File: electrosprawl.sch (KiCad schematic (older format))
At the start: 53 parts, among them J1 3.3v, J2 Conn_02x08_Odd_Even, J67 Conn_02x05_Counter_Clockwise, J7 VCC, J70 TXRX, J71 Micro_SD_Card_Det, J74 USB_B_Micro, SW1 Reset, U2 samd51p20, U5 LM1117-3.3, Y1 Crystal

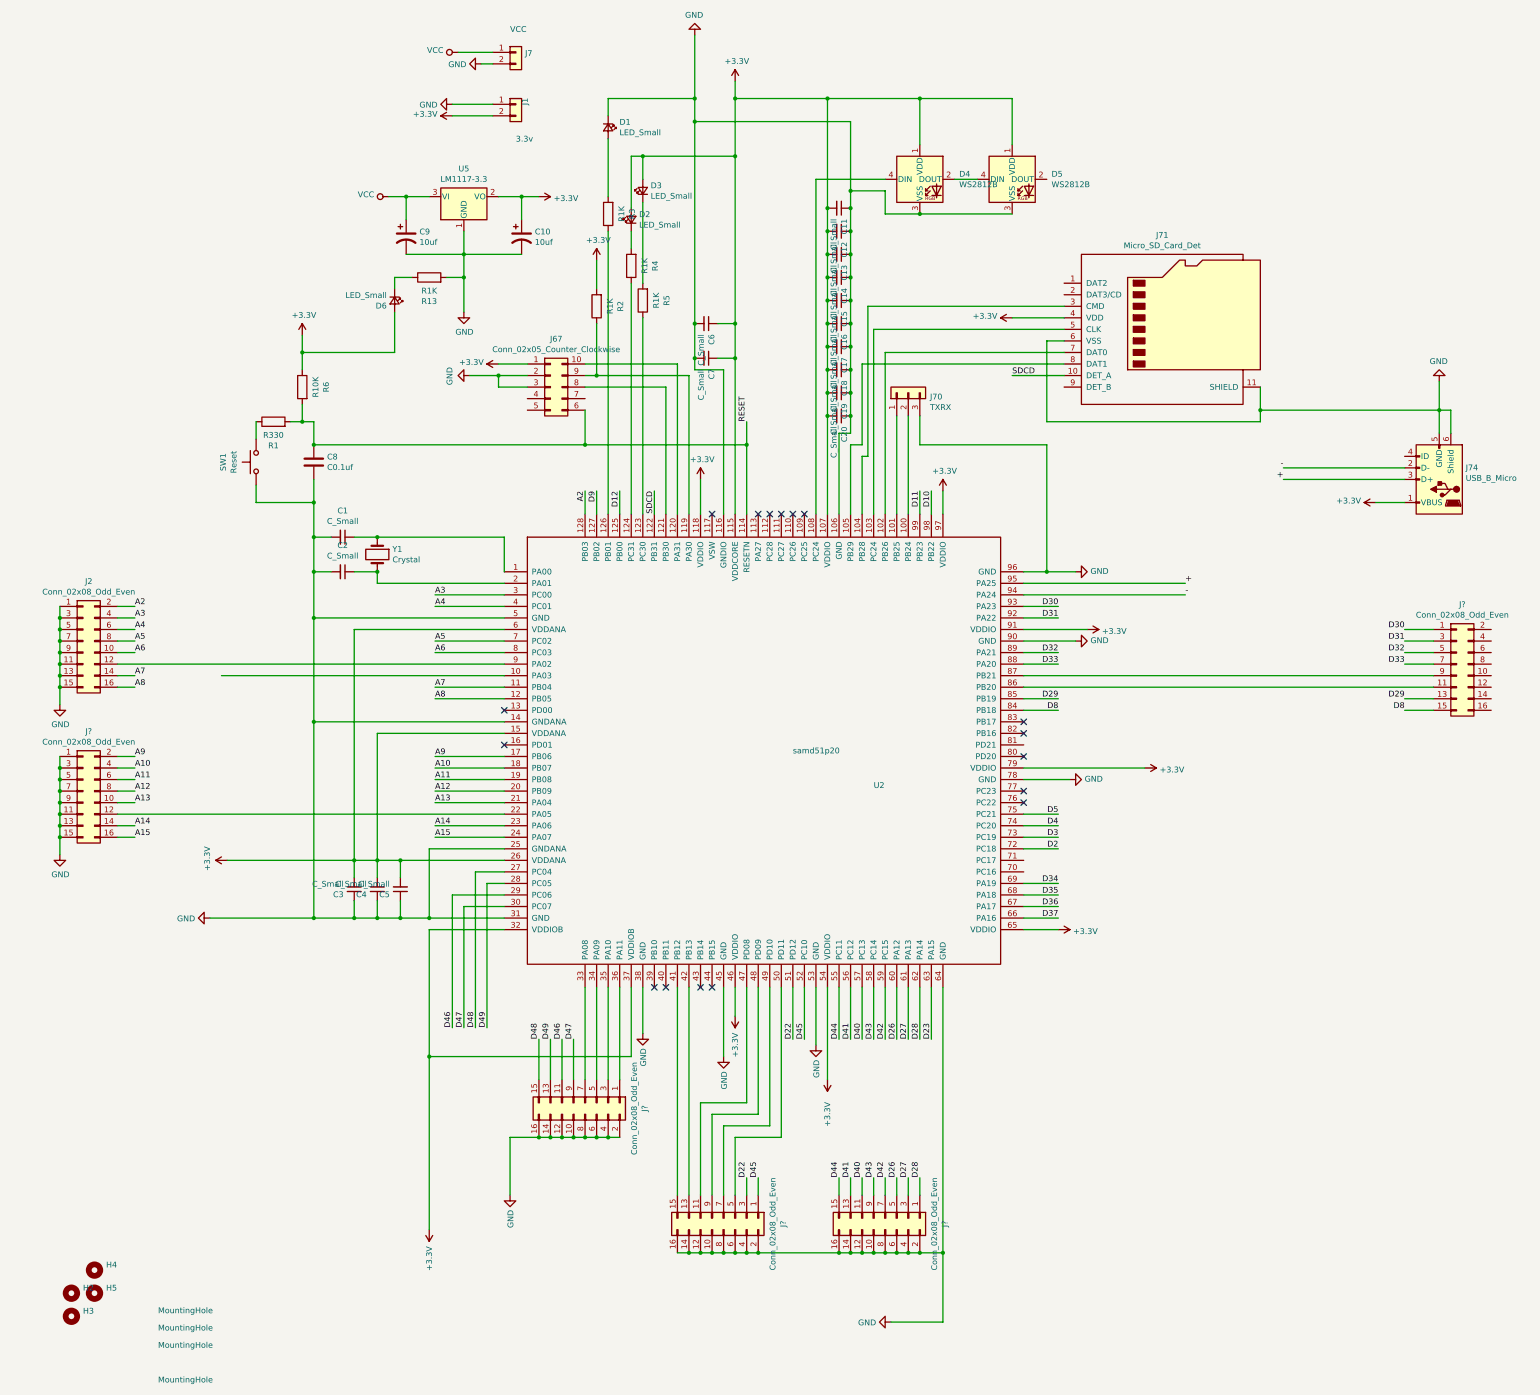
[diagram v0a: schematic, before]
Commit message: update layout
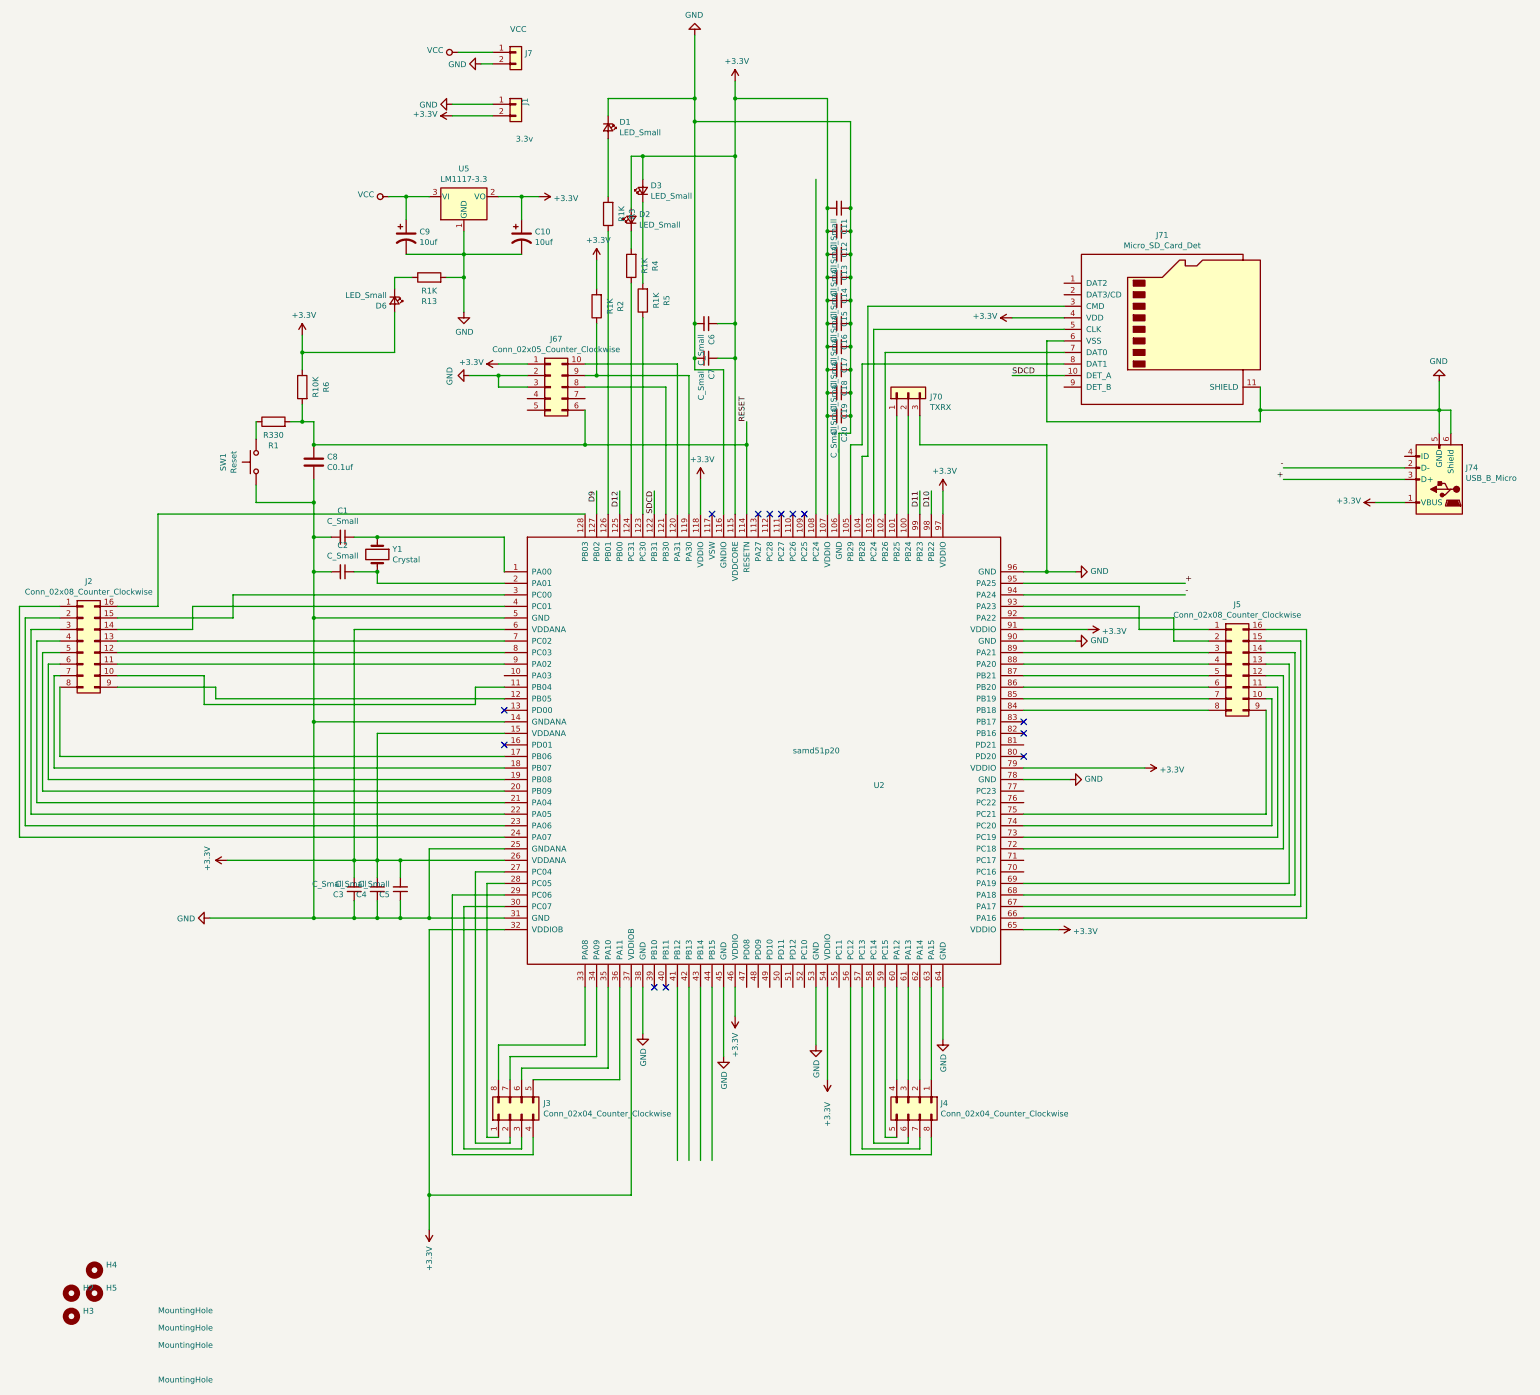
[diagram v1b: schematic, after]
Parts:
- removed D4, D5: WS2812B, LED_SMD:LED_WS2812B_PLCC4_5.0x5.0mm_P3.2mm, symbol LED:WS2812B
- removed J2, J? (x5): Conn_02x08_Odd_Even, Connector_PinHeader_2.54mm:PinHeader_2x08_P2.54mm_Vertical, symbol Connector_Generic:Conn_02x08_Odd_Even
- added J2, J5: Conn_02x08_Counter_Clockwise, Connector_PinHeader_2.54mm:PinHeader_2x08_P2.54mm_Vertical, symbol Connector_Generic:Conn_02x08_Counter_Clockwise
- added J3, J4: Conn_02x04_Counter_Clockwise, Connector_PinHeader_2.54mm:PinHeader_2x04_P2.54mm_Vertical, symbol Connector_Generic:Conn_02x04_Counter_Clockwise
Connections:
- net at U2.22 (PA05): now also J2.3 (Pin_3)
- net at U2.33 (PA08): now also J3.8 (Pin_8)
- net at U2.34 (PA09): now also J3.7 (Pin_7)
- net at U2.35 (PA10): now also J3.6 (Pin_6)
- net at U2.36 (PA11): now also J3.5 (Pin_5)
- net at U2.86 (PB20): now also J5.6 (Pin_6)
- net at U2.87 (PB21): now also J5.5 (Pin_5)
- net at U2.9 (PA02): now also J2.11 (Pin_11)
- net A10: no longer names the net of U2.18 (PB07)
- net A10: now also J2.7 (Pin_7)
- net A11: no longer names the net of U2.19 (PB08)
- net A11: now also J2.6 (Pin_6)
- net A12: no longer names the net of U2.20 (PB09)
- net A12: now also J2.5 (Pin_5)
- net A13: no longer names the net of U2.21 (PA04)
- net A13: now also J2.4 (Pin_4)
- net A14: no longer names the net of U2.23 (PA06)
- net A14: now also J2.2 (Pin_2)
- net A15: no longer names the net of U2.24 (PA07)
- net A15: now also J2.1 (Pin_1)
- net A2: no longer names the net of U2.128 (PB03)
- net A2: now also J2.16 (Pin_16)
- net A3: no longer names the net of U2.3 (PC00)
- net A3: now also J2.15 (Pin_15)
- net A4: no longer names the net of U2.4 (PC01)
- net A4: now also J2.14 (Pin_14)
- net A5: no longer names the net of U2.7 (PC02)
- net A5: now also J2.13 (Pin_13)
- net A6: no longer names the net of U2.8 (PC03)
- net A6: now also J2.12 (Pin_12)
- net A7: no longer names the net of U2.11 (PB04)
- net A7: now also J2.10 (Pin_10)
- net A8: no longer names the net of U2.12 (PB05)
- net A8: now also J2.9 (Pin_9)
- net A9: no longer names the net of U2.17 (PB06)
- net A9: now also J2.8 (Pin_8)
- net D2: no longer names the net of U2.72 (PC18)
- net D2: now also J5.12 (Pin_12)
- net D22: no longer names the net of U2.51 (PD12)
- net D23: no longer names the net of U2.63 (PA15)
- net D23: now also J4.1 (Pin_1)
- net D26: no longer names the net of U2.60 (PA12)
- net D26: now also J4.4 (Pin_4)
- net D27: no longer names the net of U2.61 (PA13)
- net D27: now also J4.3 (Pin_3)
- net D28: no longer names the net of U2.62 (PA14)
- net D28: now also J4.2 (Pin_2)
- net D29: no longer names the net of U2.85 (PB19)
- net D29: now also J5.7 (Pin_7)
- net D3: no longer names the net of U2.73 (PC19)
- net D3: now also J5.11 (Pin_11)
- net D30: no longer names the net of U2.93 (PA23)
- net D30: now also J5.1 (Pin_1)
- net D31: no longer names the net of U2.92 (PA22)
- net D31: now also J5.2 (Pin_2)
- net D32: no longer names the net of U2.89 (PA21)
- net D32: now also J5.3 (Pin_3)
- net D33: no longer names the net of U2.88 (PA20)
- net D33: now also J5.4 (Pin_4)
- net D34: no longer names the net of U2.69 (PA19)
- net D34: now also J5.13 (Pin_13)
- net D35: no longer names the net of U2.68 (PA18)
- net D35: now also J5.14 (Pin_14)
- net D36: no longer names the net of U2.67 (PA17)
- net D36: now also J5.15 (Pin_15)
- net D37: no longer names the net of U2.66 (PA16)
- net D37: now also J5.16 (Pin_16)
- net D4: no longer names the net of U2.74 (PC20)
- net D4: now also J5.10 (Pin_10)
- net D40: no longer names the net of U2.57 (PC13)
- net D40: now also J4.7 (Pin_7)
- net D41: no longer names the net of U2.56 (PC12)
- net D41: now also J4.8 (Pin_8)
- net D42: no longer names the net of U2.59 (PC15)
- net D42: now also J4.5 (Pin_5)
- net D43: no longer names the net of U2.58 (PC14)
- net D43: now also J4.6 (Pin_6)
- net D44: no longer names the net of U2.55 (PC11)
- net D45: no longer names the net of U2.52 (PC10)
- net D46: no longer names the net of U2.29 (PC06)
- net D46: now also J3.4 (Pin_4)
- net D47: no longer names the net of U2.30 (PC07)
- net D47: now also J3.3 (Pin_3)
- net D48: no longer names the net of U2.27 (PC04)
- net D48: now also J3.2 (Pin_2)
- net D49: no longer names the net of U2.28 (PC05)
- net D49: now also J3.1 (Pin_1)
- net D5: no longer names the net of U2.75 (PC21)
- net D5: now also J5.9 (Pin_9)
- net D8: no longer names the net of U2.84 (PB18)
- net D8: now also J5.8 (Pin_8)
- no-connect marks 17 -> 13

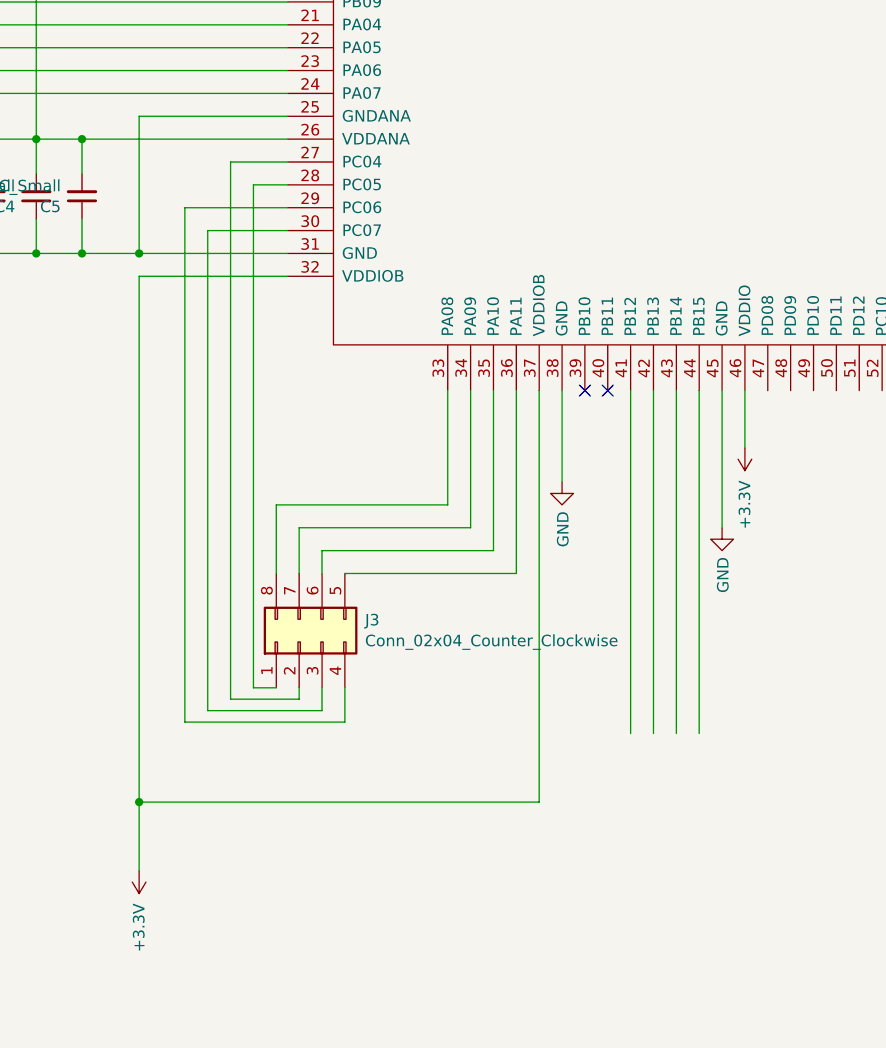
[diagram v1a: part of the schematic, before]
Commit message: update redesign
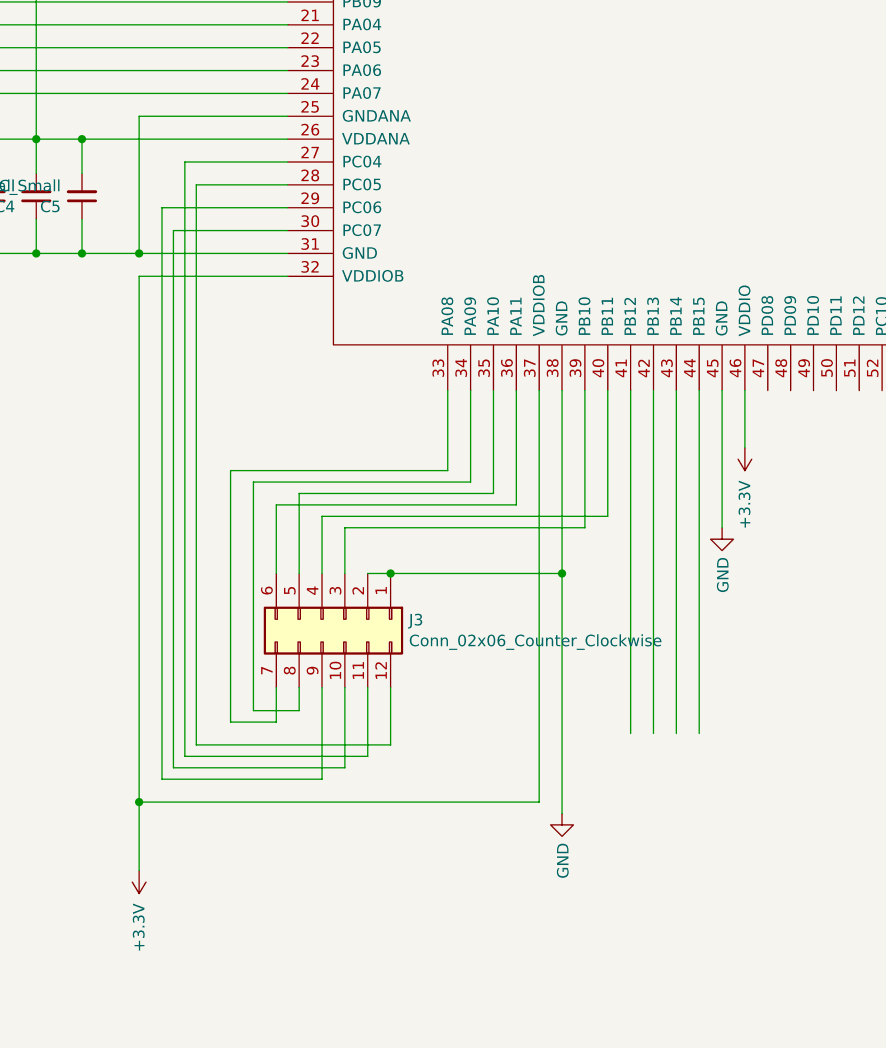
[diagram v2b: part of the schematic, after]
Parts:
- removed J3: Conn_02x04_Counter_Clockwise, Connector_PinHeader_2.54mm:PinHeader_2x04_P2.54mm_Vertical, symbol Connector_Generic:Conn_02x04_Counter_Clockwise
- added J3: Conn_02x06_Counter_Clockwise, Connector_PinHeader_2.54mm:PinHeader_2x06_P2.54mm_Vertical, symbol Connector_Generic:Conn_02x06_Counter_Clockwise
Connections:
- net GND: now also J3.1 (Pin_1), J3.2 (Pin_2)
- net at U2.27 (PC04): now also J3.11 (Pin_11)
- net at U2.28 (PC05): now also J3.12 (Pin_12)
- net at U2.29 (PC06): now also J3.9 (Pin_9)
- net at U2.30 (PC07): now also J3.10 (Pin_10)
- net at U2.33 (PA08): now also J3.7 (Pin_7)
- net at U2.34 (PA09): now also J3.8 (Pin_8)
- net at U2.35 (PA10): now also J3.5 (Pin_5)
- net at U2.36 (PA11): now also J3.6 (Pin_6)
- net at U2.39 (PB10): now also J3.3 (Pin_3)
- net at U2.40 (PB11): now also J3.4 (Pin_4)
- no-connect marks 13 -> 11
